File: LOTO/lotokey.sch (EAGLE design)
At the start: 14 parts

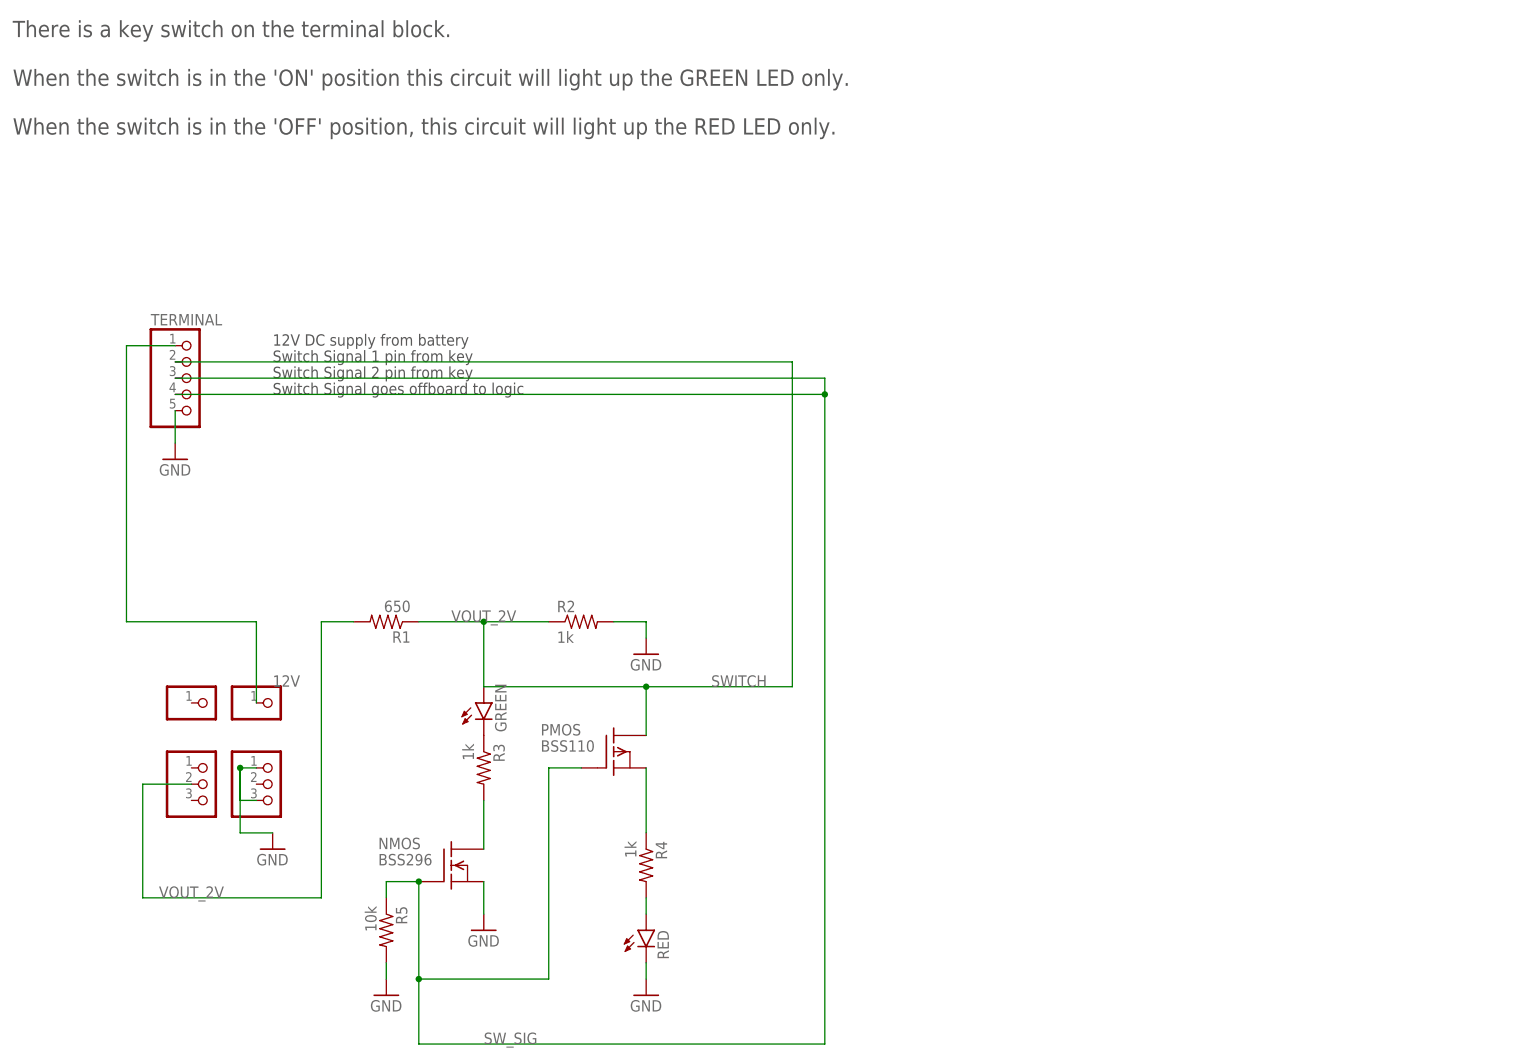
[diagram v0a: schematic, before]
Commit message: adding isolated ps
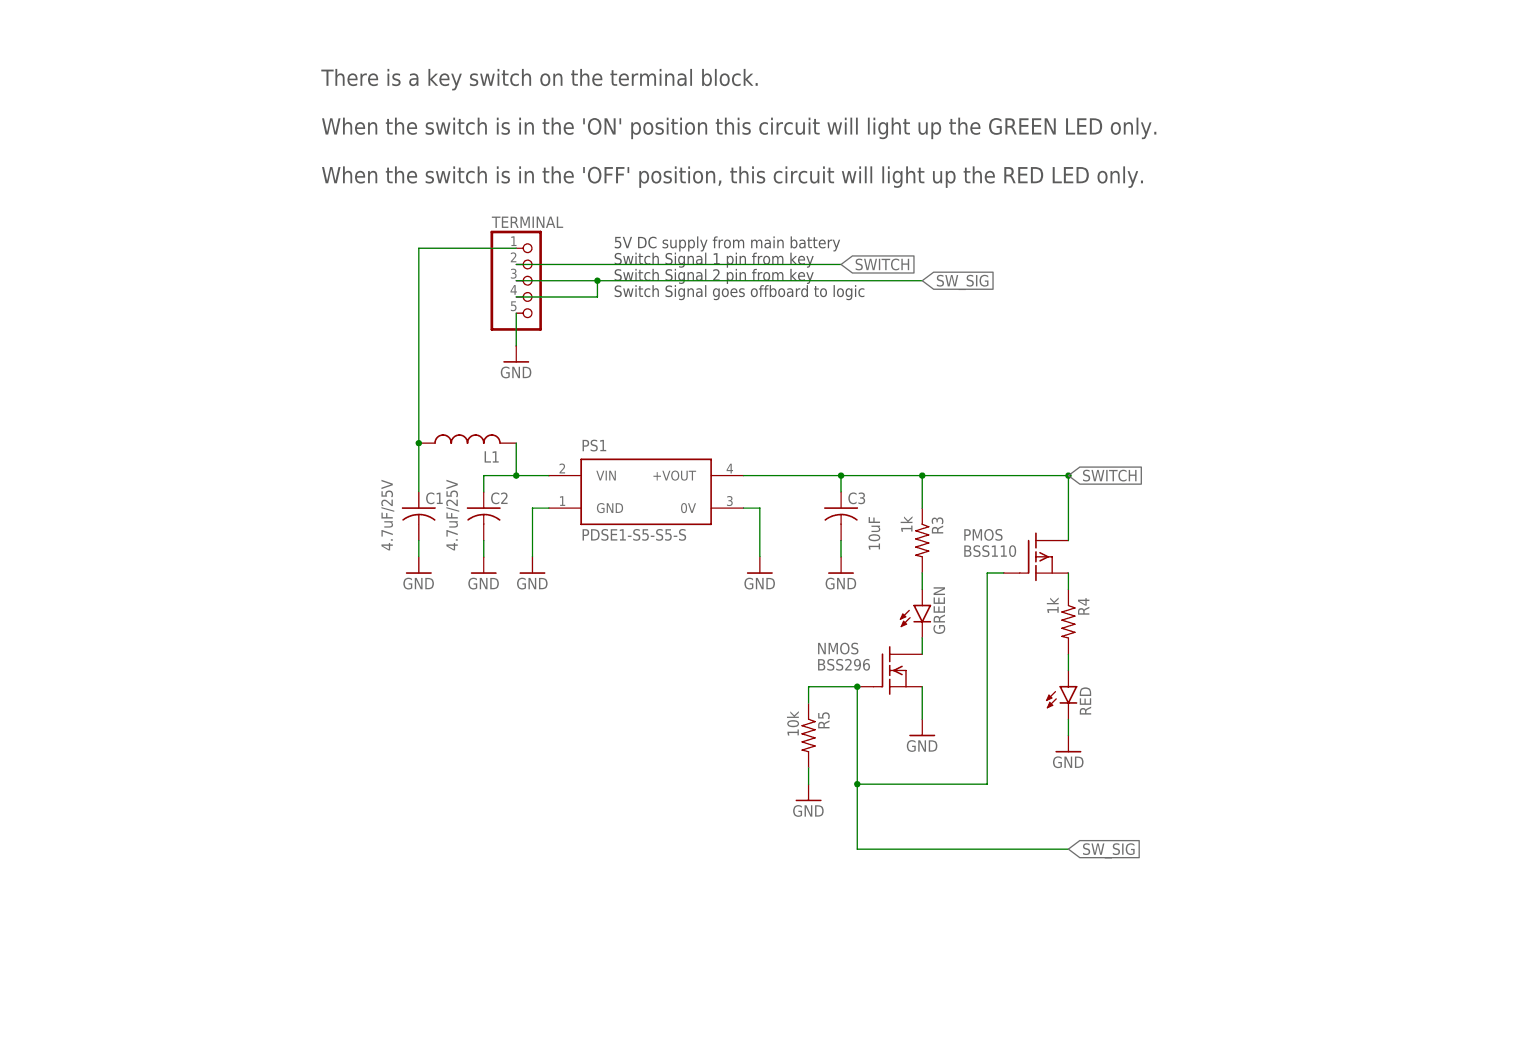
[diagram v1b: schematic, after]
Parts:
- removed JP1, JP2: (no value), pinhead:PINHD-1X1
- removed JP3, JP4: (no value), pinhead:PINHD-1X3
- removed R1: 650, rcl:R-US_0204/7
- removed R2: 1k, rcl:R-US_0204/7
- added C1, C2: 4.7uF/25V, rcl:C-US050-025X075
- added C3: 10uF, rcl:C-US050-025X075
- added L1: (no value), rcl:L-US0204/5
- added PS1: PDSE1-S5-S5-S, PDSE1-S5-S5-S:PDSE1-S5-S5-S
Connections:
- removed net N$5: NMOS.D, R3.2
- removed net VOUT_2V: JP4.2, R1.2
- new net N$1: C2.1, L1.2, PS1.VIN
- new net N$3: GREEN.C, NMOS.D
- net 12V: now also C1.1, L1.1; no longer JP1.1
- net GND: now also C1.2, C2.2, C3.2, PS1.0V, PS1.GND; no longer JP3.1, JP3.3, R2.2
- net N$4: now also GREEN.A, R3.2; no longer GREEN.C, R3.1
- net SWITCH: now also C3.1, PS1.+VOUT, R3.1; no longer GREEN.A, R1.1, R2.1
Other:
- note added: "5V DC supply from main battery"
- note removed: "12V DC supply from battery"
- moved on the sheet: GREEN, NMOS, PMOS, R3, R4, R5, RED, TERMINAL

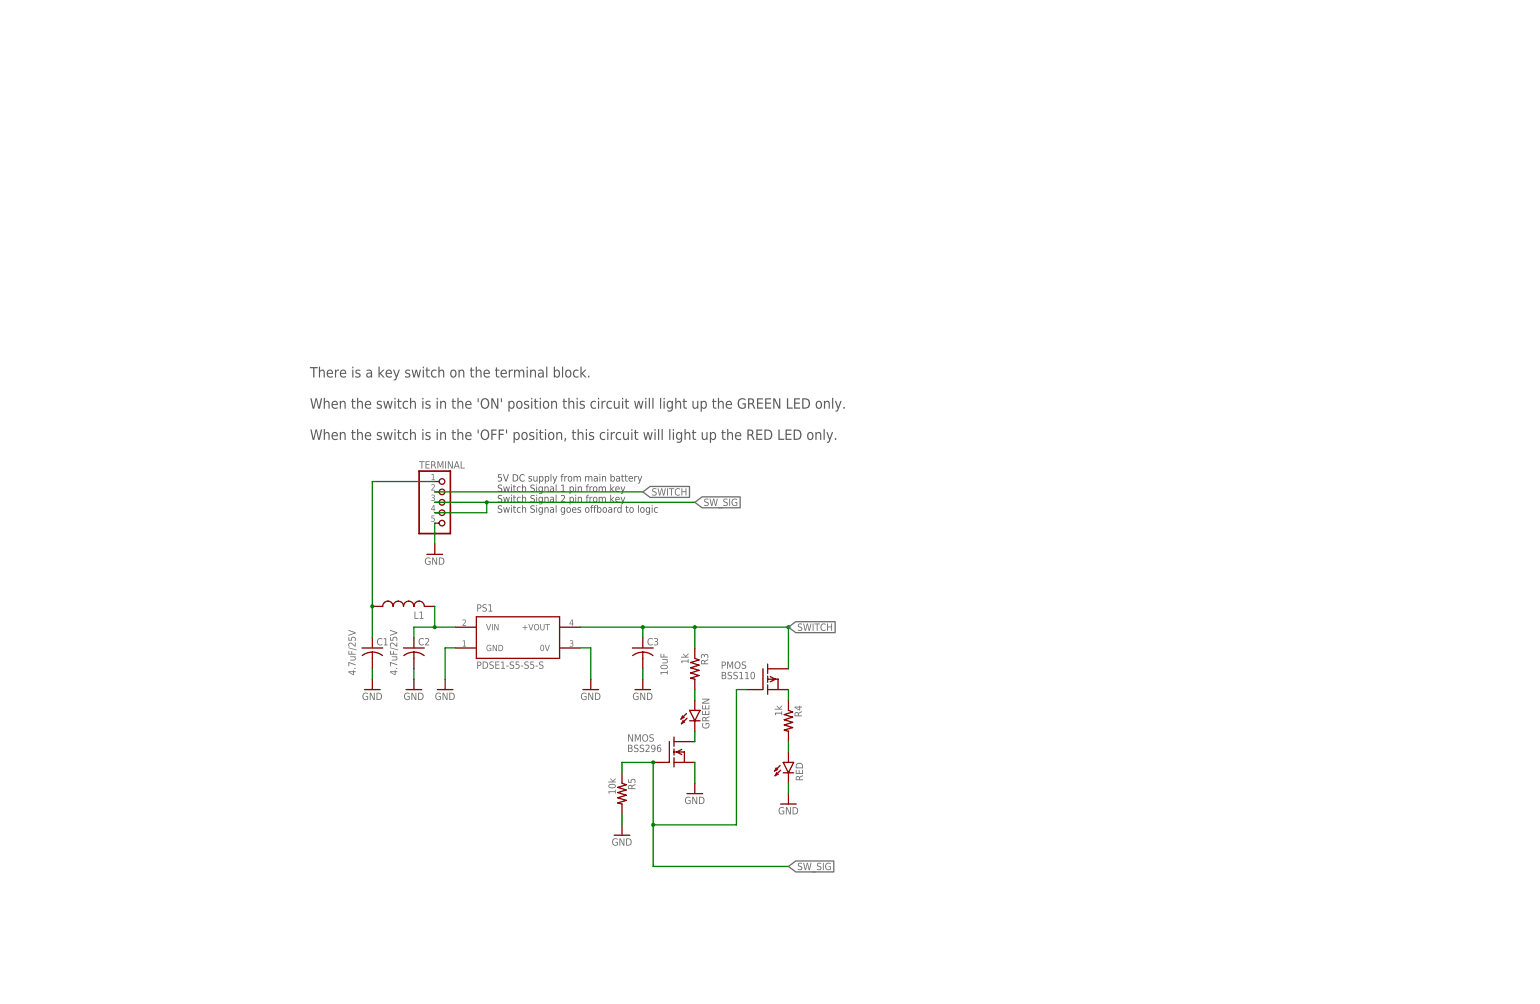
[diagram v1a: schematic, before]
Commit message: Updated LOTO boards
Added LOTO housing outline.  Added logic for POE power and gate trigger. Added more circuit protection and power isolation.
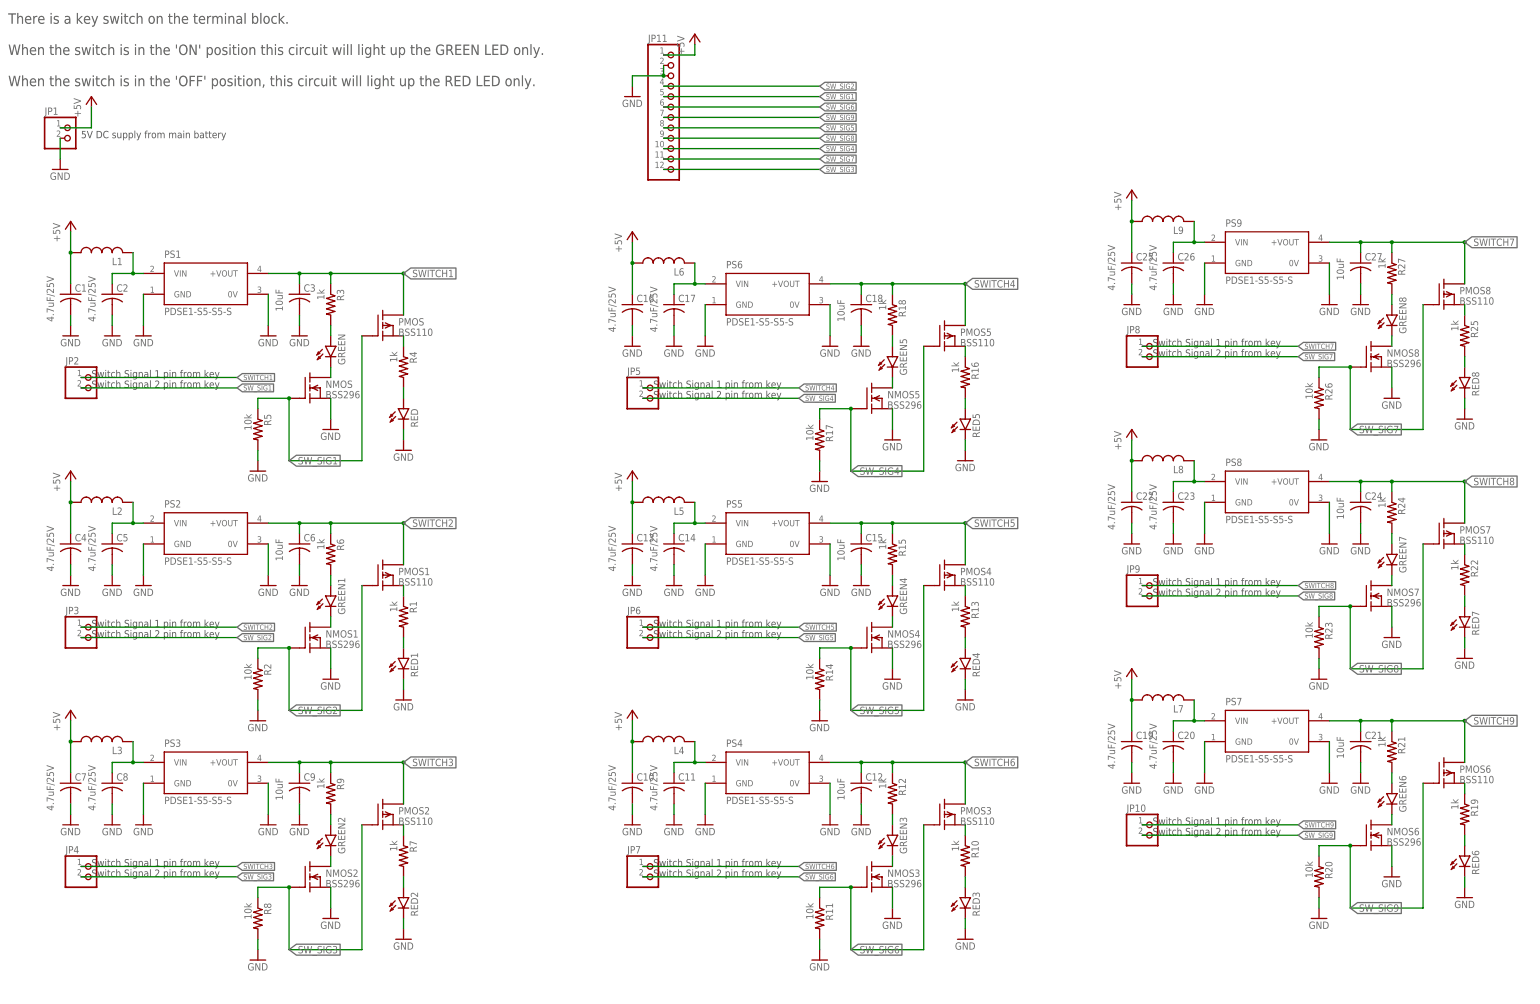
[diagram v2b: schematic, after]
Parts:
- removed TERMINAL: (no value), 5mmtermblock:PINHD-1X5
- added C10, C11, C13, C14, C16, C17, C19, C20, C22, C23, C25, C26, C4, C5, C7, C8: 4.7uF/25V, rcl:C-US050-025X075
- added C12, C15, C18, C21, C24, C27, C6, C9: 10uF, rcl:C-US050-025X075
- added GREEN1, GREEN2, GREEN3, GREEN4, GREEN5, GREEN6, GREEN7, GREEN8, RED1, RED2, RED3, RED4, RED5, RED6, RED7, RED8: TLLR4400, led:TLLR4400
- added JP1, JP10, JP2, JP3, JP4, JP5, JP6, JP7, JP8, JP9: (no value), pinhead:PINHD-1X2
- added JP11: (no value), pinhead:PINHD-1X12
- added L2, L3, L4, L5, L6, L7, L8, L9: (no value), rcl:L-US0204/5
- added NMOS1, NMOS2, NMOS3, NMOS4, NMOS5, NMOS6, NMOS7, NMOS8: BSS296, transistor-fet:BSS296
- added PMOS1, PMOS2, PMOS3, PMOS4, PMOS5, PMOS6, PMOS7, PMOS8: BSS110, transistor-fet:BSS110
- added PS2, PS3, PS4, PS5, PS6, PS7, PS8, PS9: PDSE1-S5-S5-S, PDSE1-S5-S5-S:PDSE1-S5-S5-S
- added R1, R10, R12, R13, R15, R16, R18, R19, R21, R22, R24, R25, R27, R6, R7, R9: 1k, rcl:R-US_0204/7
- added R11, R14, R17, R2, R20, R23, R26, R8: 10k, rcl:R-US_0204/7
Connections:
- removed net 12V: C1.1, L1.1, TERMINAL.1
- removed net SWITCH: C3.1, PMOS.D, PS1.+VOUT, R3.1, TERMINAL.2
- removed net SW_SIG: NMOS.G, PMOS.G, R5.1, TERMINAL.3, TERMINAL.4
- new net +5V: C1.1, C10.1, C13.1, C16.1, C19.1, C22.1, C25.1, C4.1, C7.1, JP1.1, JP11.1, L1.1, L2.1, L3.1, L4.1, L5.1, L6.1, L7.1, L8.1, L9.1
- new net N$10: GREEN1.A, R6.2
- new net N$11: R7.2, RED2.A
- new net N$12: PMOS2.S, R7.1
- new net N$13: C8.1, L3.2, PS3.VIN
- new net N$14: GREEN2.C, NMOS2.D
- new net N$15: GREEN2.A, R9.2
- new net N$16: R10.2, RED3.A
- new net N$17: PMOS3.S, R10.1
- new net N$18: C11.1, L4.2, PS4.VIN
- new net N$19: GREEN3.C, NMOS3.D
- new net N$2: R1.2, RED1.A
- new net N$20: GREEN3.A, R12.2
- new net N$21: R13.2, RED4.A
- new net N$22: PMOS4.S, R13.1
- new net N$23: C14.1, L5.2, PS5.VIN
- new net N$24: GREEN4.C, NMOS4.D
- new net N$25: GREEN4.A, R15.2
- new net N$26: R16.2, RED5.A
- new net N$27: PMOS5.S, R16.1
- new net N$28: C17.1, L6.2, PS6.VIN
- new net N$29: GREEN5.C, NMOS5.D
- new net N$30: GREEN5.A, R18.2
- new net N$31: R19.2, RED6.A
- new net N$32: PMOS6.S, R19.1
- new net N$33: C20.1, L7.2, PS7.VIN
- new net N$34: GREEN6.C, NMOS6.D
- new net N$35: GREEN6.A, R21.2
- new net N$36: R22.2, RED7.A
- new net N$37: PMOS7.S, R22.1
- new net N$38: C23.1, L8.2, PS8.VIN
- new net N$39: GREEN7.C, NMOS7.D
- new net N$40: GREEN7.A, R24.2
- new net N$41: R25.2, RED8.A
- new net N$42: PMOS8.S, R25.1
- new net N$43: C26.1, L9.2, PS9.VIN
- new net N$44: GREEN8.C, NMOS8.D
- new net N$45: GREEN8.A, R27.2
- new net N$5: PMOS1.S, R1.1
- new net N$6: C5.1, L2.2, PS2.VIN
- new net N$7: GREEN1.C, NMOS1.D
- new net SWITCH1: C3.1, JP2.1, PMOS.D, PS1.+VOUT, R3.1
- new net SWITCH2: C6.1, JP3.1, PMOS1.D, PS2.+VOUT, R6.1
- new net SWITCH3: C9.1, JP4.1, PMOS2.D, PS3.+VOUT, R9.1
- new net SWITCH4: C18.1, JP5.1, PMOS5.D, PS6.+VOUT, R18.1
- new net SWITCH5: C15.1, JP6.1, PMOS4.D, PS5.+VOUT, R15.1
- new net SWITCH6: C12.1, JP7.1, PMOS3.D, PS4.+VOUT, R12.1
- new net SWITCH7: C27.1, JP8.1, PMOS8.D, PS9.+VOUT, R27.1
- new net SWITCH8: C24.1, JP9.1, PMOS7.D, PS8.+VOUT, R24.1
- new net SWITCH9: C21.1, JP10.1, PMOS6.D, PS7.+VOUT, R21.1
- new net SW_SIG1: JP11.5, JP2.2, NMOS.G, PMOS.G, R5.1
- new net SW_SIG2: JP11.4, JP3.2, NMOS1.G, PMOS1.G, R2.1
- new net SW_SIG3: JP11.12, JP4.2, NMOS2.G, PMOS2.G, R8.1
- new net SW_SIG4: JP11.10, JP5.2, NMOS5.G, PMOS5.G, R17.1
- new net SW_SIG5: JP11.8, JP6.2, NMOS4.G, PMOS4.G, R14.1
- new net SW_SIG6: JP11.6, JP7.2, NMOS3.G, PMOS3.G, R11.1
- new net SW_SIG7: JP11.11, JP8.2, NMOS8.G, PMOS8.G, R26.1
- new net SW_SIG8: JP11.9, JP9.2, NMOS7.G, PMOS7.G, R23.1
- new net SW_SIG9: JP10.2, JP11.7, NMOS6.G, PMOS6.G, R20.1
- net GND: now also C10.2, C11.2, C12.2, C13.2, C14.2, C15.2, C16.2, C17.2, C18.2, C19.2, C20.2, C21.2, C22.2, C23.2, C24.2, C25.2, C26.2, C27.2, C4.2, C5.2, C6.2, C7.2, C8.2, C9.2, JP1.2, JP11.2, JP11.3, NMOS1.S, NMOS2.S, NMOS3.S, NMOS4.S, NMOS5.S, NMOS6.S, NMOS7.S, NMOS8.S, PS2.0V, PS2.GND, PS3.0V, PS3.GND, PS4.0V, PS4.GND, PS5.0V, PS5.GND, PS6.0V, PS6.GND, PS7.0V, PS7.GND, PS8.0V, PS8.GND, PS9.0V, PS9.GND, R11.2, R14.2, R17.2, R2.2, R20.2, R23.2, R26.2, R8.2, RED1.C, RED2.C, RED3.C, RED4.C, RED5.C, RED6.C, RED7.C, RED8.C; no longer TERMINAL.5
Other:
- note removed: "Switch Signal goes offboard to logic"
- moved on the sheet: C1, C2, C3, GREEN, L1, NMOS, PMOS, PS1, R3, R4, R5, RED
